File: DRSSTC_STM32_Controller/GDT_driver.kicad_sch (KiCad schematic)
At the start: 36 parts, among them IC1 UCC27282DR, IC2 UCC27282DR, J5 Screw_Terminal_01x02, Q1 QM6006D, Q2 QM6006D, Q3 QM6006D, Q4 QM6006D

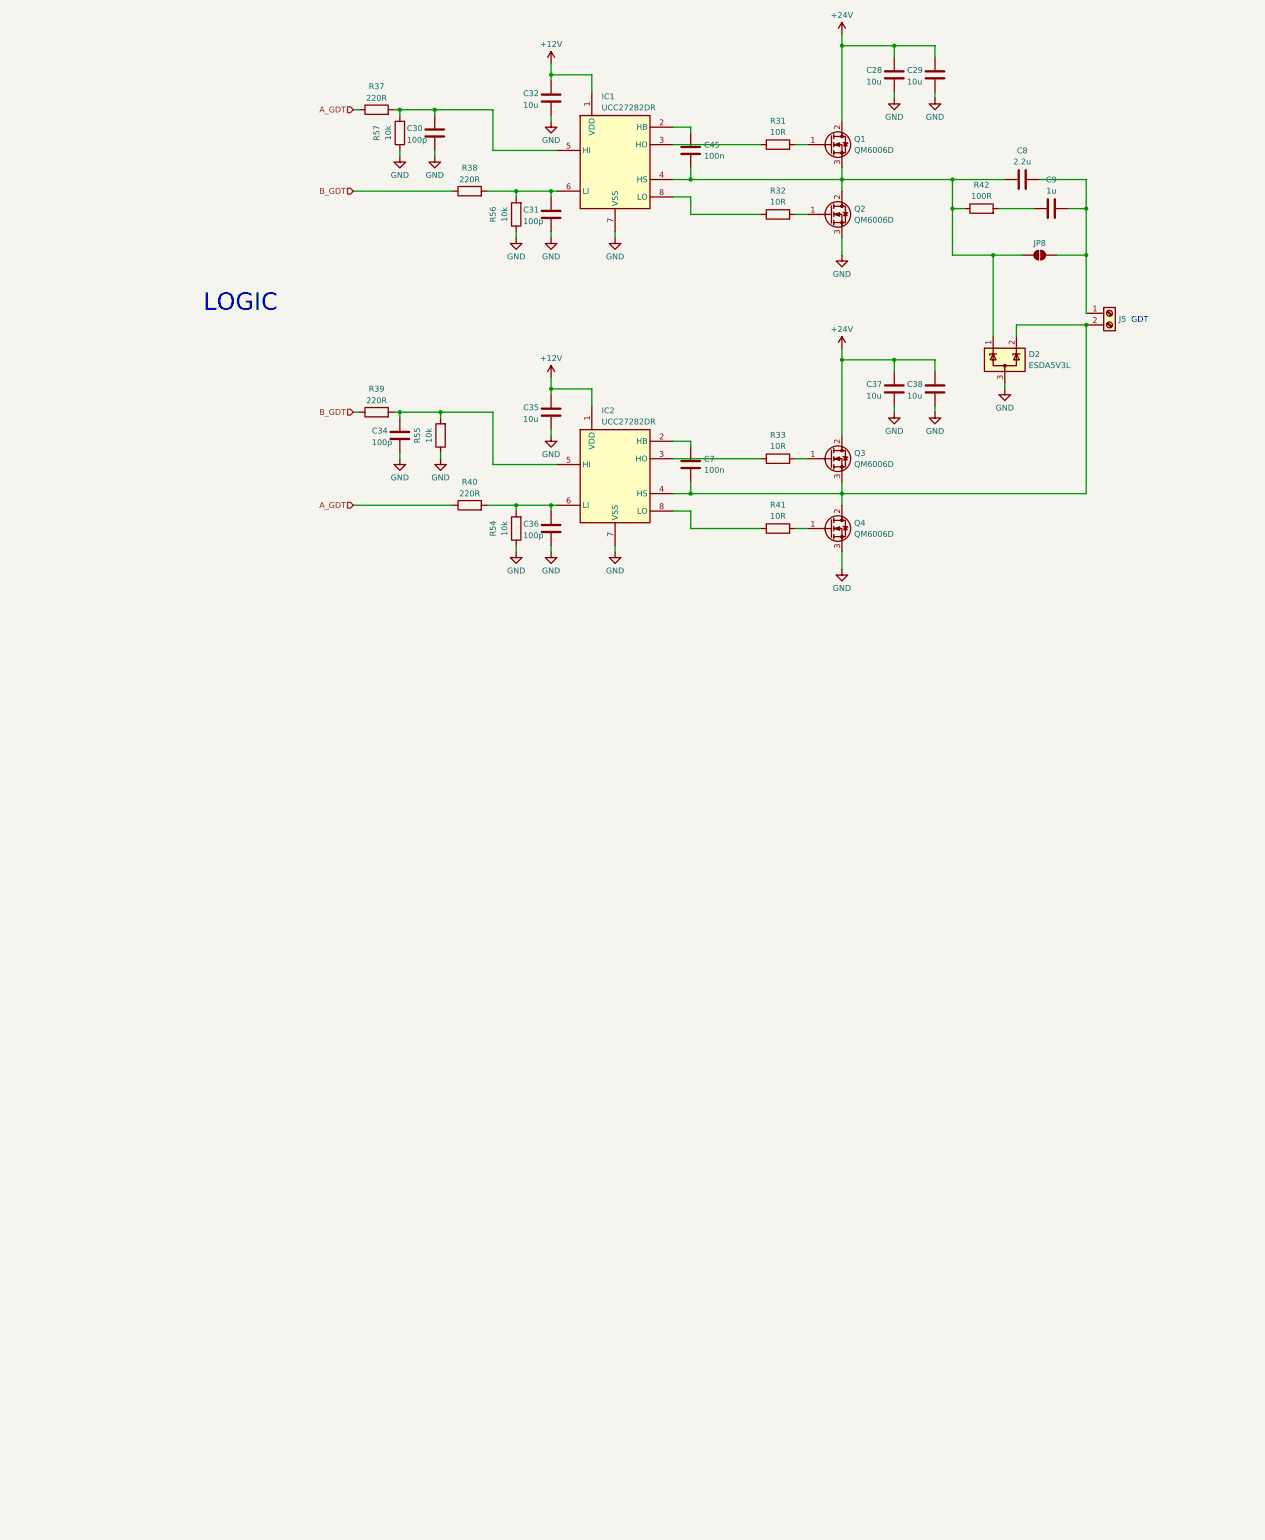
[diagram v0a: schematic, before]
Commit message: update conroller schematics
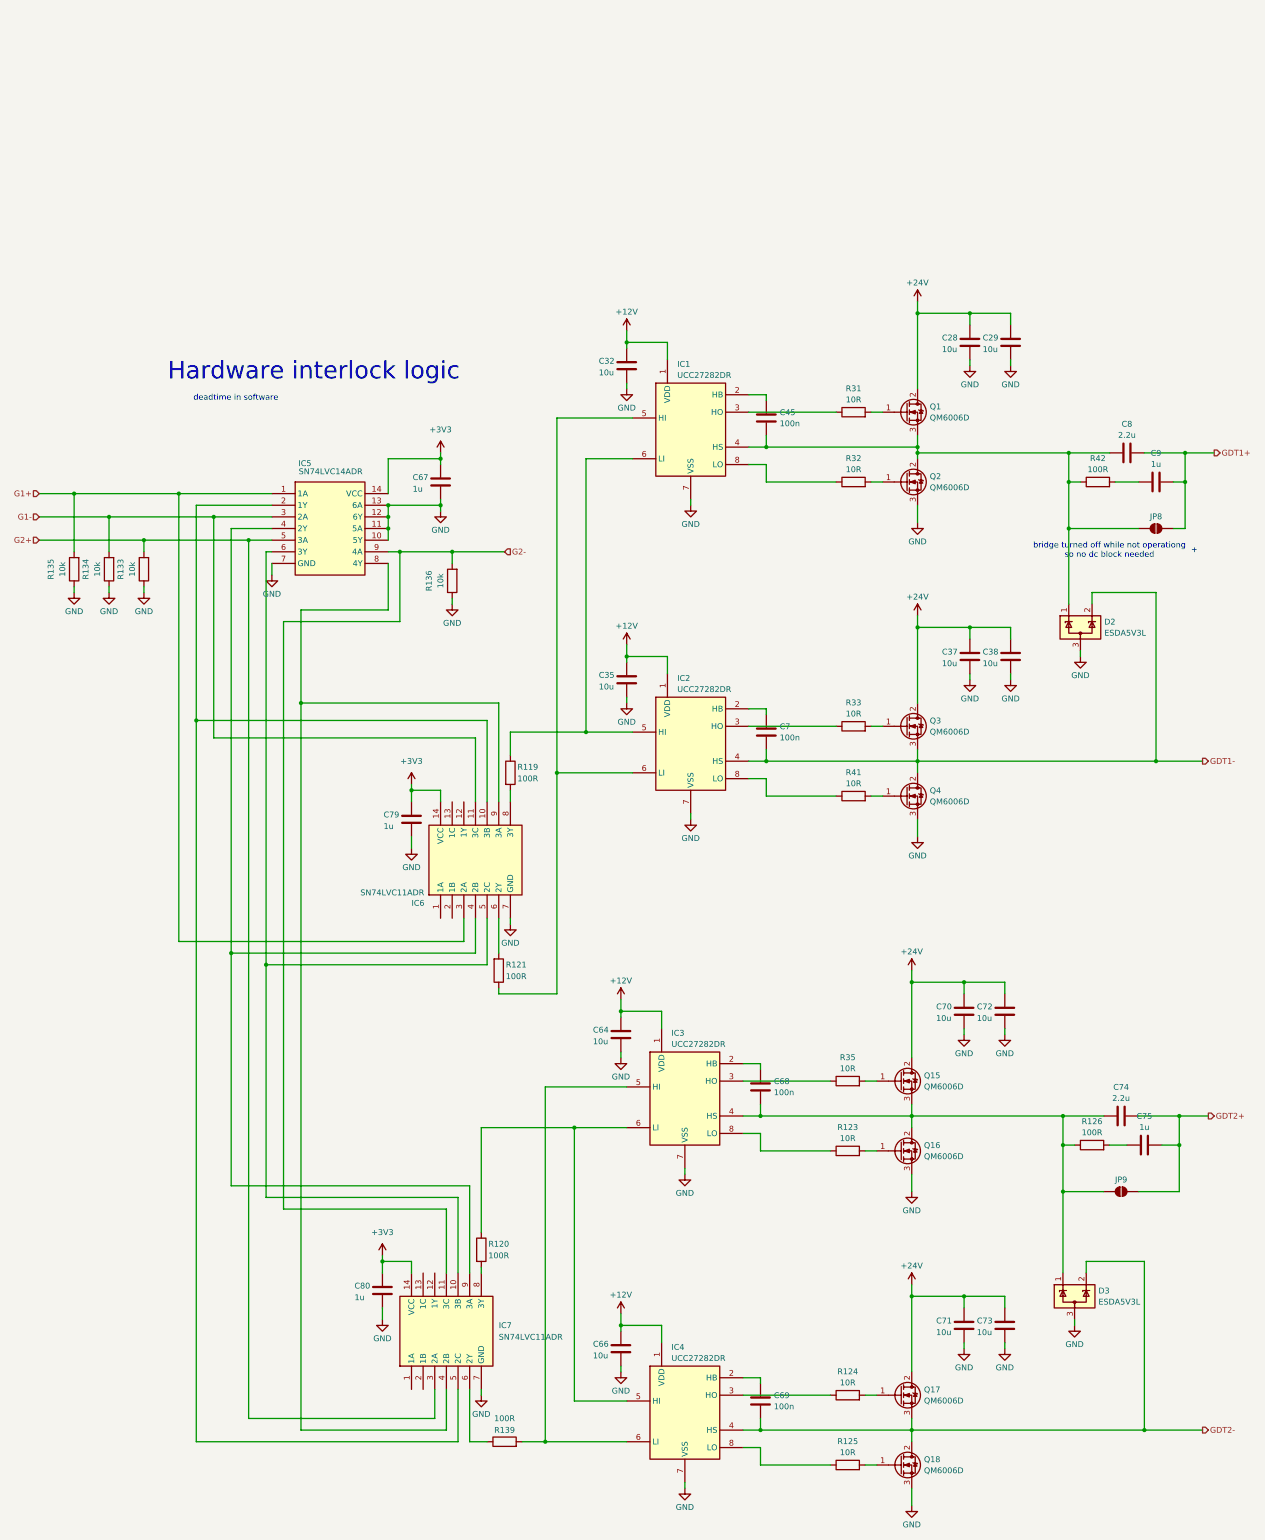
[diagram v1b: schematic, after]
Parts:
- removed C30, C31, C34, C36: 100p, Capacitor_SMD:C_0805_2012Metric, symbol Device:C
- removed J5: Screw_Terminal_01x02, TerminalBlock_Altech:Altech_AK100_1x02_P5.00mm, symbol Connector:Screw_Terminal_01x02
- removed R37, R38, R39, R40: 220R, Resistor_SMD:R_0805_2012Metric, symbol Device:R
- removed R54, R55, R56, R57: 10k, Resistor_SMD:R_0805_2012Metric, symbol Device:R
- added C64, C66, C70, C71, C72, C73: 10u, Capacitor_SMD:C_0805_2012Metric, symbol Device:C
- added C67, C79, C80: 1u, Capacitor_SMD:C_0805_2012Metric, symbol Device:C
- added C68, C69: 100n, symbol Device:C
- added C74: 2.2u, symbol Device:C
- added C75: 1u, symbol Device:C
- added D3: ESDA5V3L, Package_TO_SOT_SMD:SOT-23-3, symbol Power_Protection:ESDA5V3L
- added IC3, IC4: UCC27282DR, SOIC127P600X175-8N, symbol UCC27282DR:UCC27282DR
- added IC5: SN74LVC14ADR, Library:SOIC127P600X175-14N, symbol SN74LVC14ADR:SN74LVC14ADR
- added IC6, IC7: SN74LVC11ADR, Library:SOIC127P600X175-14N, symbol Library:SN74LVC11ADR
- added JP9: SolderJumper_2_Open, Jumper:SolderJumper-2_P1.3mm_Open_RoundedPad1.0x1.5mm, symbol Jumper:SolderJumper_2_Open
- added Q15, Q16, Q17, Q18: QM6006D, Package_TO_SOT_SMD:TO-252-2, symbol Transistor_FET:QM6006D
- added R119, R120, R121, R126, R139: 100R, Resistor_SMD:R_0805_2012Metric, symbol Device:R
- added R123, R124, R125, R35: 10R, Resistor_SMD:R_0805_2012Metric, symbol Device:R
- added R133, R134, R135, R136: 10k, Resistor_SMD:R_0805_2012Metric, symbol Device:R
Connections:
- net +12V: now also C64.1, C66.1, IC3.1 (VDD), IC4.1 (VDD)
- net +24V: now also C70.1, C71.1, C72.1, C73.1, Q15.2 (D), Q17.2 (D)
- net GND: now also C64.2, C66.2, C67.2, C70.2, C71.2, C72.2, C73.2, C79.2, C80.2, D3.3 (A), IC3.7 (VSS), IC4.7 (VSS), IC5.10 (5Y), IC5.11 (5A), IC5.12 (6Y), IC5.13 (6A), IC5.7 (GND), IC6.7 (GND), IC7.7 (GND), Q16.3 (S), Q18.3 (S), R133.1, R134.1, R135.1, R136.1
- net GDT1+: now reaches C8.2, C9.2, JP8.1 (A)
- net GDT1-: now reaches C7.2, D2.2 (K), IC2.4 (HS), Q3.3 (S), Q4.2 (D)
- net at IC1.6 (LI): now also IC2.5 (HI), R119.1
- net at IC1.5 (HI): now also IC2.6 (LI), R121.1
- new net: IC4.3 (HO), R124.1
- new net: Q17.1 (G), R124.2
- new net: C68.2, C74.1, D3.1 (K), IC3.4 (HS), JP9.2 (B), Q15.3 (S), Q16.2 (D), R126.1
- new net: C68.1, IC3.2 (HB)
- new net: IC3.3 (HO), R35.1
- new net: IC3.5 (HI), IC4.6 (LI), R139.2
- new net: IC3.6 (LI), IC4.5 (HI), R120.1
- new net: IC3.8 (LO), R123.1
- new net: Q18.1 (G), R125.2
- new net: IC4.8 (LO), R125.1
- new net: IC5.2 (1Y), IC6.10 (3B), IC7.5 (2C)
- new net: IC5.4 (2Y), IC6.4 (2B), IC7.9 (3A)
- new net: IC5.6 (3Y), IC6.5 (2C), IC7.10 (3B)
- new net: IC5.8 (4Y), IC6.9 (3A), IC7.4 (2B)
- new net: IC6.6 (2Y), R121.2
- new net: Q15.1 (G), R35.2
- new net: IC6.8 (3Y), R119.2
- new net: IC7.8 (3Y), R120.2
- new net: C75.1, R126.2
- new net: Q16.1 (G), R123.2
- new net: C69.1, IC4.2 (HB)
- new net: IC7.6 (2Y), R139.1
- new net +3V3: C67.1, C79.1, C80.1, IC5.14 (VCC), IC6.14 (VCC), IC7.14 (VCC)
- new net G1+: IC5.1 (1A), IC6.3 (2A), R135.2
- new net G1-: IC5.3 (2A), IC6.11 (3C), R134.2
- new net G2+: IC5.5 (3A), IC7.3 (2A), R133.2
- new net G2-: IC5.9 (4A), IC7.11 (3C), R136.2
- new net GDT2+: C74.2, C75.2, JP9.1 (A)
- new net GDT2-: C69.2, D3.2 (K), IC4.4 (HS), Q17.3 (S), Q18.2 (D)
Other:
- note added: "+"
- note added: "Hardware interlock logic"
- note added: "bridge turned off while not operationg so no dc block needed"
- note added: "deadtime in software"
- note removed: "GDT"
- note removed: "LOGIC"
- moved on the sheet: C28, C29, C32, C35, C37, C38, C45, C7, C8, C9, D2, IC1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

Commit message: assign footprints
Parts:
- C45, C68, C69: footprint (none) -> Capacitor_SMD:C_0603_1608Metric
- C67, C79, C80: footprint Capacitor_SMD:C_0805_2012Metric -> Capacitor_SMD:C_0603_1608Metric
- C7: footprint (none) -> Capacitor_SMD:C_0201_0603Metric
- C74, C75, C8, C9: footprint (none) -> Capacitor_THT:C_Axial_L12.0mm_D7.5mm_P15.00mm_Horizontal
- IC1, IC2, IC3, IC4: footprint SOIC127P600X175-8N -> Library:SOIC127P600X175-8N
- R119, R120, R121, R133, R134, R135, R136, R139: footprint Resistor_SMD:R_0805_2012Metric -> Resistor_SMD:R_0603_1608Metric
- R126, R42: footprint Resistor_SMD:R_0805_2012Metric -> Resistor_THT:R_Axial_DIN0309_L9.0mm_D3.2mm_P12.70mm_Horizontal
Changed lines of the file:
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@@
 			)
 		)
-		(property "Footprint" ""
+		(property "Footprint" "Capacitor_THT:C_Axial_L12.0mm_D7.5mm_P15.00mm_Horizontal"
 			(at 261.62 120.9548 0)
 			(hide yes)
@@
 			)
 		)
-		(property "Footprint" "SOIC127P600X175-8N"
+		(property "Footprint" "Library:SOIC127P600X175-8N"
 			(at 171.45 210.49 0)
 			(hide yes)
@@
 			)
 		)
-		(property "Footprint" "Resistor_SMD:R_0805_2012Metric"
+		(property "Footprint" "Resistor_THT:R_Axial_DIN0309_L9.0mm_D3.2mm_P12.70mm_Horizontal"
 			(at 251.46 130.048 90)
 			(hide yes)
@@
 			)
 		)
-		(property "Footprint" "Resistor_SMD:R_0805_2012Metric"
+		(property "Footprint" "Resistor_SMD:R_0603_1608Metric"
 			(at 112.268 149.86 90)
 			(hide yes)
@@
 			)
 		)
-		(property "Footprint" "Capacitor_SMD:C_0805_2012Metric"
+		(property "Footprint" "Capacitor_SMD:C_0603_1608Metric"
 			(at 108.9152 132.08 0)
 			(hide yes)
@@
 			)
 		)
-		(property "Footprint" "SOIC127P600X175-8N"
+		(property "Footprint" "Library:SOIC127P600X175-8N"
 			(at 170.18 356.54 0)
 			(hide yes)
@@
 			)
 		)
-		(property "Footprint" "Resistor_SMD:R_0805_2012Metric"
+		(property "Footprint" "Resistor_SMD:R_0603_1608Metric"
 			(at 37.338 147.32 90)
 			(hide yes)
@@
 			)
 		)
-		(property "Footprint" "SOIC127P600X175-8N"
+		(property "Footprint" "Library:SOIC127P600X175-8N"
 			(at 171.45 279.07 0)
 			(hide yes)
@@
 			)
 		)
-		(property "Footprint" "Capacitor_SMD:C_0805_2012Metric"
+		(property "Footprint" "Capacitor_SMD:C_0603_1608Metric"
 			(at 102.5652 205.74 0)
 			(hide yes)
@@
 			)
 		)
-		(property "Footprint" "Resistor_SMD:R_0805_2012Metric"
+		(property "Footprint" "Resistor_SMD:R_0603_1608Metric"
 			(at 29.718 147.32 90)
 			(hide yes)
@@
 			)
 		)
-		(property "Footprint" "Resistor_SMD:R_0805_2012Metric"
+		(property "Footprint" "Resistor_SMD:R_0603_1608Metric"
 			(at 118.872 234.95 90)
 			(hide yes)
@@
 			)
 		)
-		(property "Footprint" "Resistor_SMD:R_0805_2012Metric"
+		(property "Footprint" "Resistor_SMD:R_0603_1608Metric"
 			(at 44.958 147.32 90)
 			(hide yes)
@@
 			)
 		)
-		(property "Footprint" "Resistor_SMD:R_0805_2012Metric"
+		(property "Footprint" "Resistor_SMD:R_0603_1608Metric"
 			(at 115.062 295.91 90)
 			(hide yes)
@@
 			)
 		)
-		(property "Footprint" ""
+		(property "Footprint" "Capacitor_THT:C_Axial_L12.0mm_D7.5mm_P15.00mm_Horizontal"
 			(at 260.35 265.7348 0)
 			(hide yes)
@@
 			)
 		)
-		(property "Footprint" "Resistor_SMD:R_0805_2012Metric"
+		(property "Footprint" "Resistor_SMD:R_0603_1608Metric"
 			(at 121.412 191.77 90)
 			(hide yes)
@@
 			)
 		)
-		(property "Footprint" ""
+		(property "Footprint" "Capacitor_THT:C_Axial_L12.0mm_D7.5mm_P15.00mm_Horizontal"
 			(at 265.43 272.0848 0)
 			(hide yes)
@@
 			)
 		)
-		(property "Footprint" ""
+		(property "Footprint" "Capacitor_SMD:C_0603_1608Metric"
 			(at 178.7652 264.16 0)
 			(hide yes)
@@
 			)
 		)
-		(property "Footprint" "Capacitor_SMD:C_0805_2012Metric"
+		(property "Footprint" "Capacitor_SMD:C_0603_1608Metric"
 			(at 96.2152 308.61 0)
 			(hide yes)
@@
 			)
 		)
-		(property "Footprint" ""
+		(property "Footprint" "Capacitor_SMD:C_0201_0603Metric"
 			(at 180.0352 186.69 0)
 			(hide yes)
@@
 			)
 		)
-		(property "Footprint" "SOIC127P600X175-8N"
+		(property "Footprint" "Library:SOIC127P600X175-8N"
 			(at 170.18 425.12 0)
 			(hide yes)
@@
 			)
 		)
-		(property "Footprint" ""
+		(property "Footprint" "Capacitor_THT:C_Axial_L12.0mm_D7.5mm_P15.00mm_Horizontal"
 			(at 267.97 127.3048 0)
 			(hide yes)
@@
 			)
 		)
-		(property "Footprint" ""
+		(property "Footprint" "Capacitor_SMD:C_0603_1608Metric"
 			(at 180.0352 118.11 0)
 			(hide yes)
@@
 			)
 		)
-		(property "Footprint" "Resistor_SMD:R_0805_2012Metric"
+		(property "Footprint" "Resistor_SMD:R_0603_1608Metric"
 			(at 121.92 339.598 90)
 			(hide yes)
@@
 			)
 		)
-		(property "Footprint" ""
+		(property "Footprint" "Capacitor_SMD:C_0603_1608Metric"
 			(at 178.7652 332.74 0)
 			(hide yes)
@@
 			)
 		)
-		(property "Footprint" "Resistor_SMD:R_0805_2012Metric"
+		(property "Footprint" "Resistor_THT:R_Axial_DIN0309_L9.0mm_D3.2mm_P12.70mm_Horizontal"
 			(at 250.19 274.828 90)
 			(hide yes)
